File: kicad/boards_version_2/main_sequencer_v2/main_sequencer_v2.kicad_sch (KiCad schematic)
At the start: 33 parts

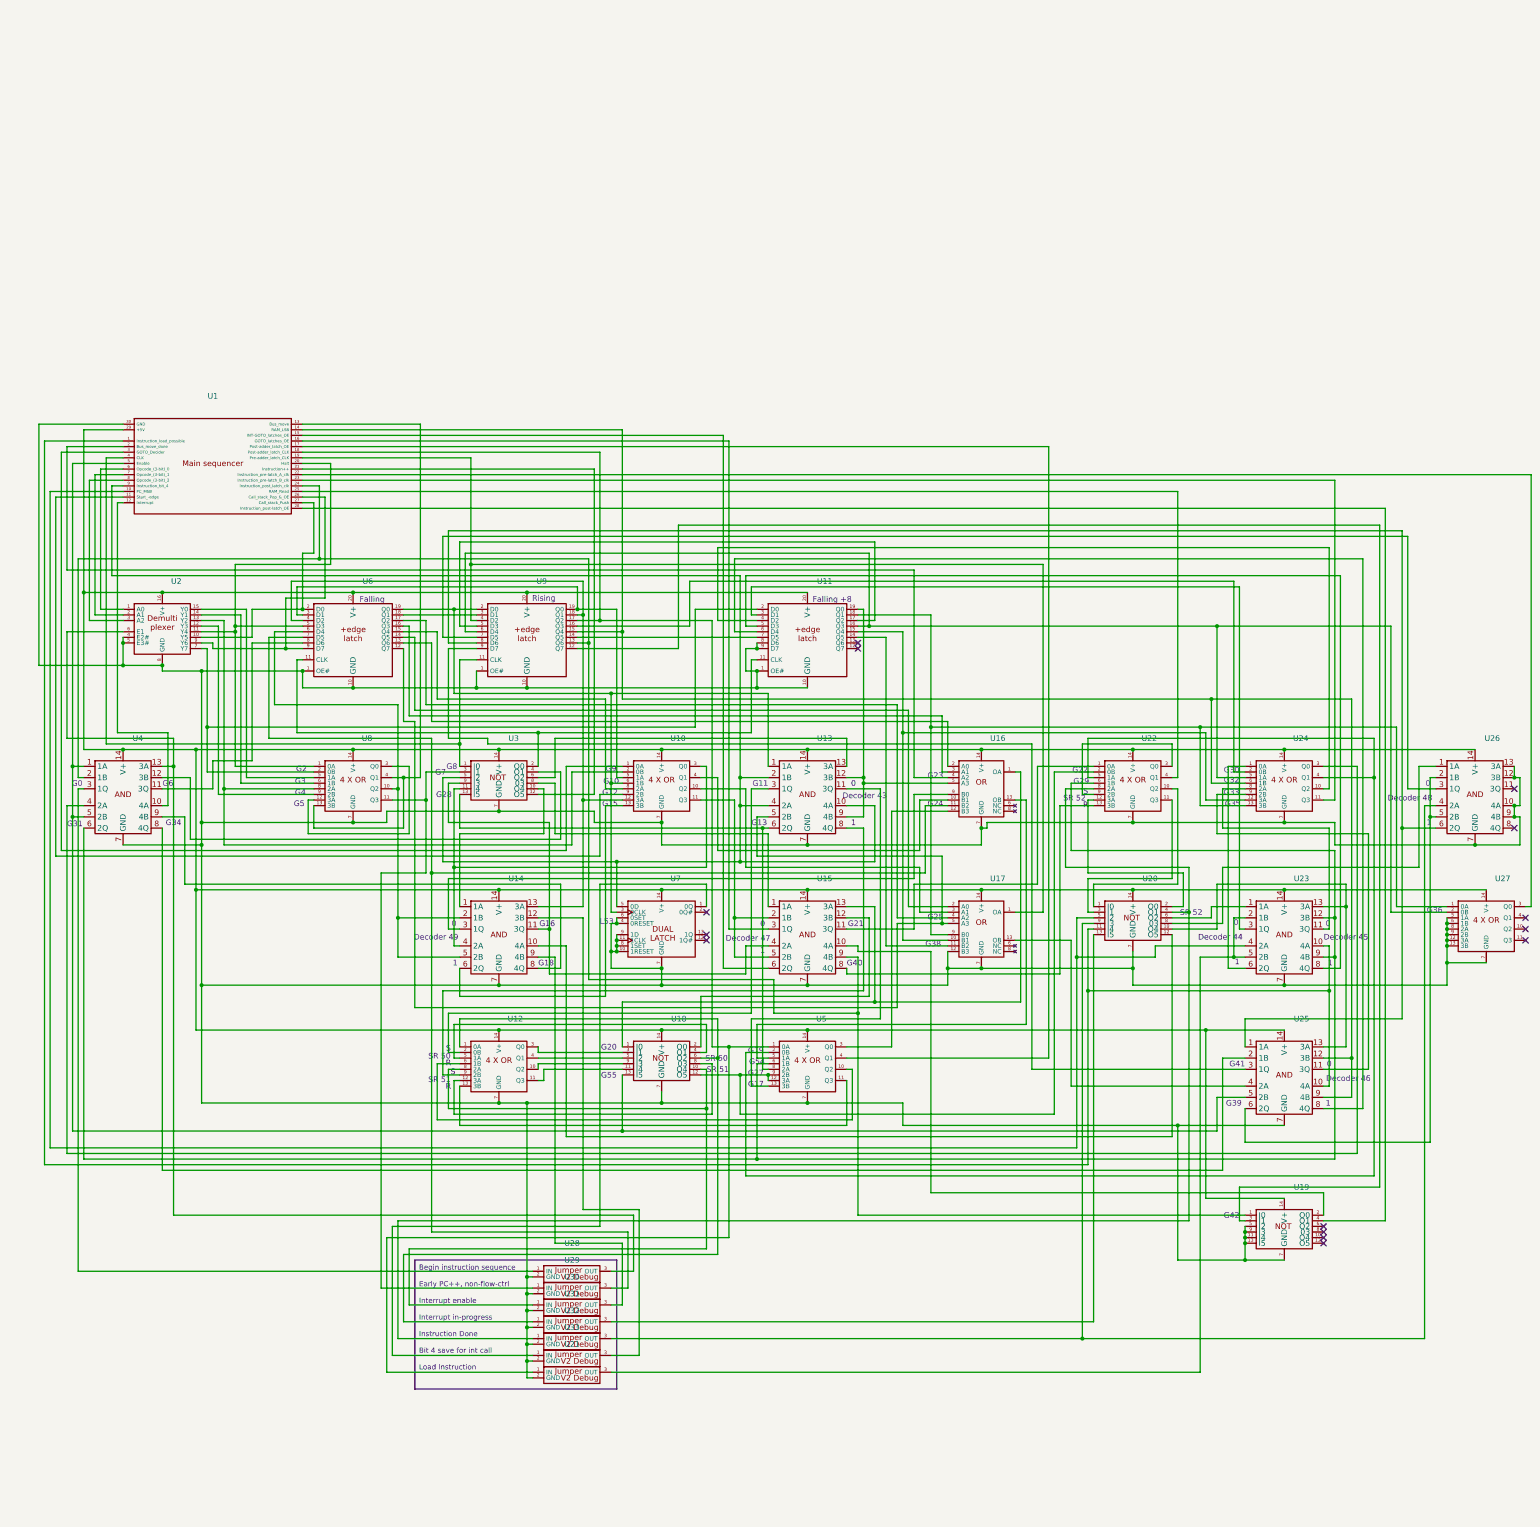
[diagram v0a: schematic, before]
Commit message: Debug figured out and work on ctrl unit main
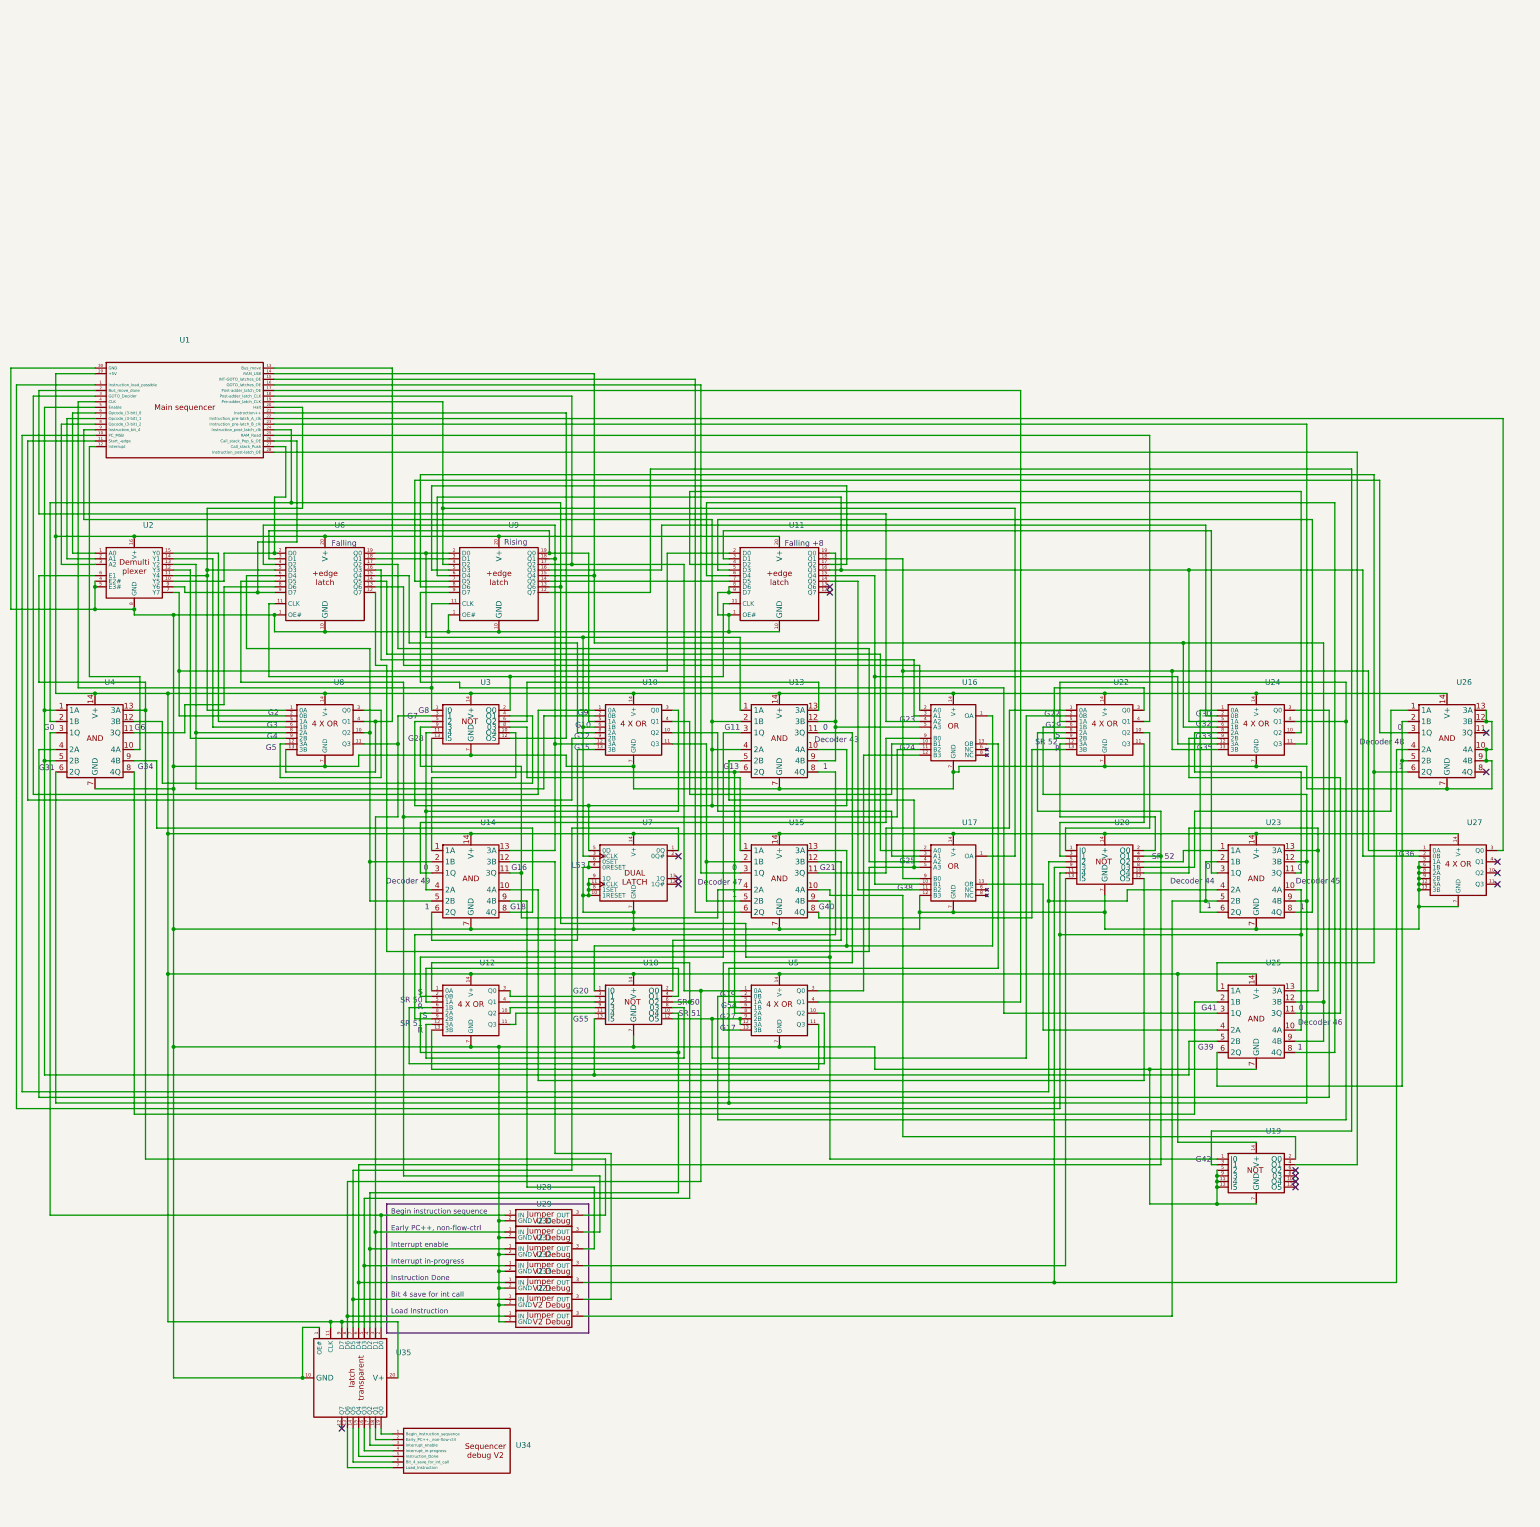
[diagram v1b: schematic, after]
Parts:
- added U34: ~, Connector_PinHeader_2.54mm:PinHeader_2x04_P2.54mm_Vertical, symbol custom_symbol_lib:debug_v2_sequencer
- added U35: ~, Package_DIP:DIP-20_W7.62mm, symbol custom_symbol_lib:8_bit_transparent_latch
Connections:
- net at U12.8 (2A), U18.10 (O4), U30.1 (IN): now also U35.4 (D2)
- net at U1.30 (GND), U10.7 (GND), U11.1 (OE#)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: now also U35.1 (OE#), U35.10 (GND)
- net at U33.1 (IN), U7.1 (0Q): now also U35.7 (D5)
- net at U1.29 (+5V), U10.14 (V+), U11.20 (V+)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: now also U35.11 (CLK), U35.20 (V+), U35.9 (D7)
- net at U28.1 (IN), U4.3 (1Q): now also U35.2 (D0)
- net at U12.1 (0A), U18.6 (O2), U31.1 (IN): now also U35.5 (D3)
- net at U29.1 (IN), U3.3 (I1), U8.11 (Q3): now also U35.3 (D1)
- net at U20.4 (O1), U22.8 (2A), U32.1 (IN): now also U35.6 (D4)
- net at U1.18 (Post-adder_latch_CLK), U21.1 (IN), U5.1 (0A)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: now also U35.8 (D6)
- new net: U34.1 (Begin_instruction_sequence), U35.19 (Q0)
- new net: U34.2 (Early_PC++,_non-flow-ctrl), U35.18 (Q1)
- new net: U34.3 (Interrupt_enable), U35.17 (Q2)
- new net: U34.4 (Interrupt_in-progress), U35.16 (Q3)
- new net: U34.5 (Instruction_Done), U35.15 (Q4)
- new net: U34.6 (Bit_4_save_for_int_call), U35.14 (Q5)
- new net: U34.7 (Load_Instruction), U35.13 (Q6)
- no-connect marks 14 -> 15
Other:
- moved on the sheet: U1, U10, U11, U12, U13, U14, U15, U16, U17, U18, U19, U2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

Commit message: Work mostly on bus
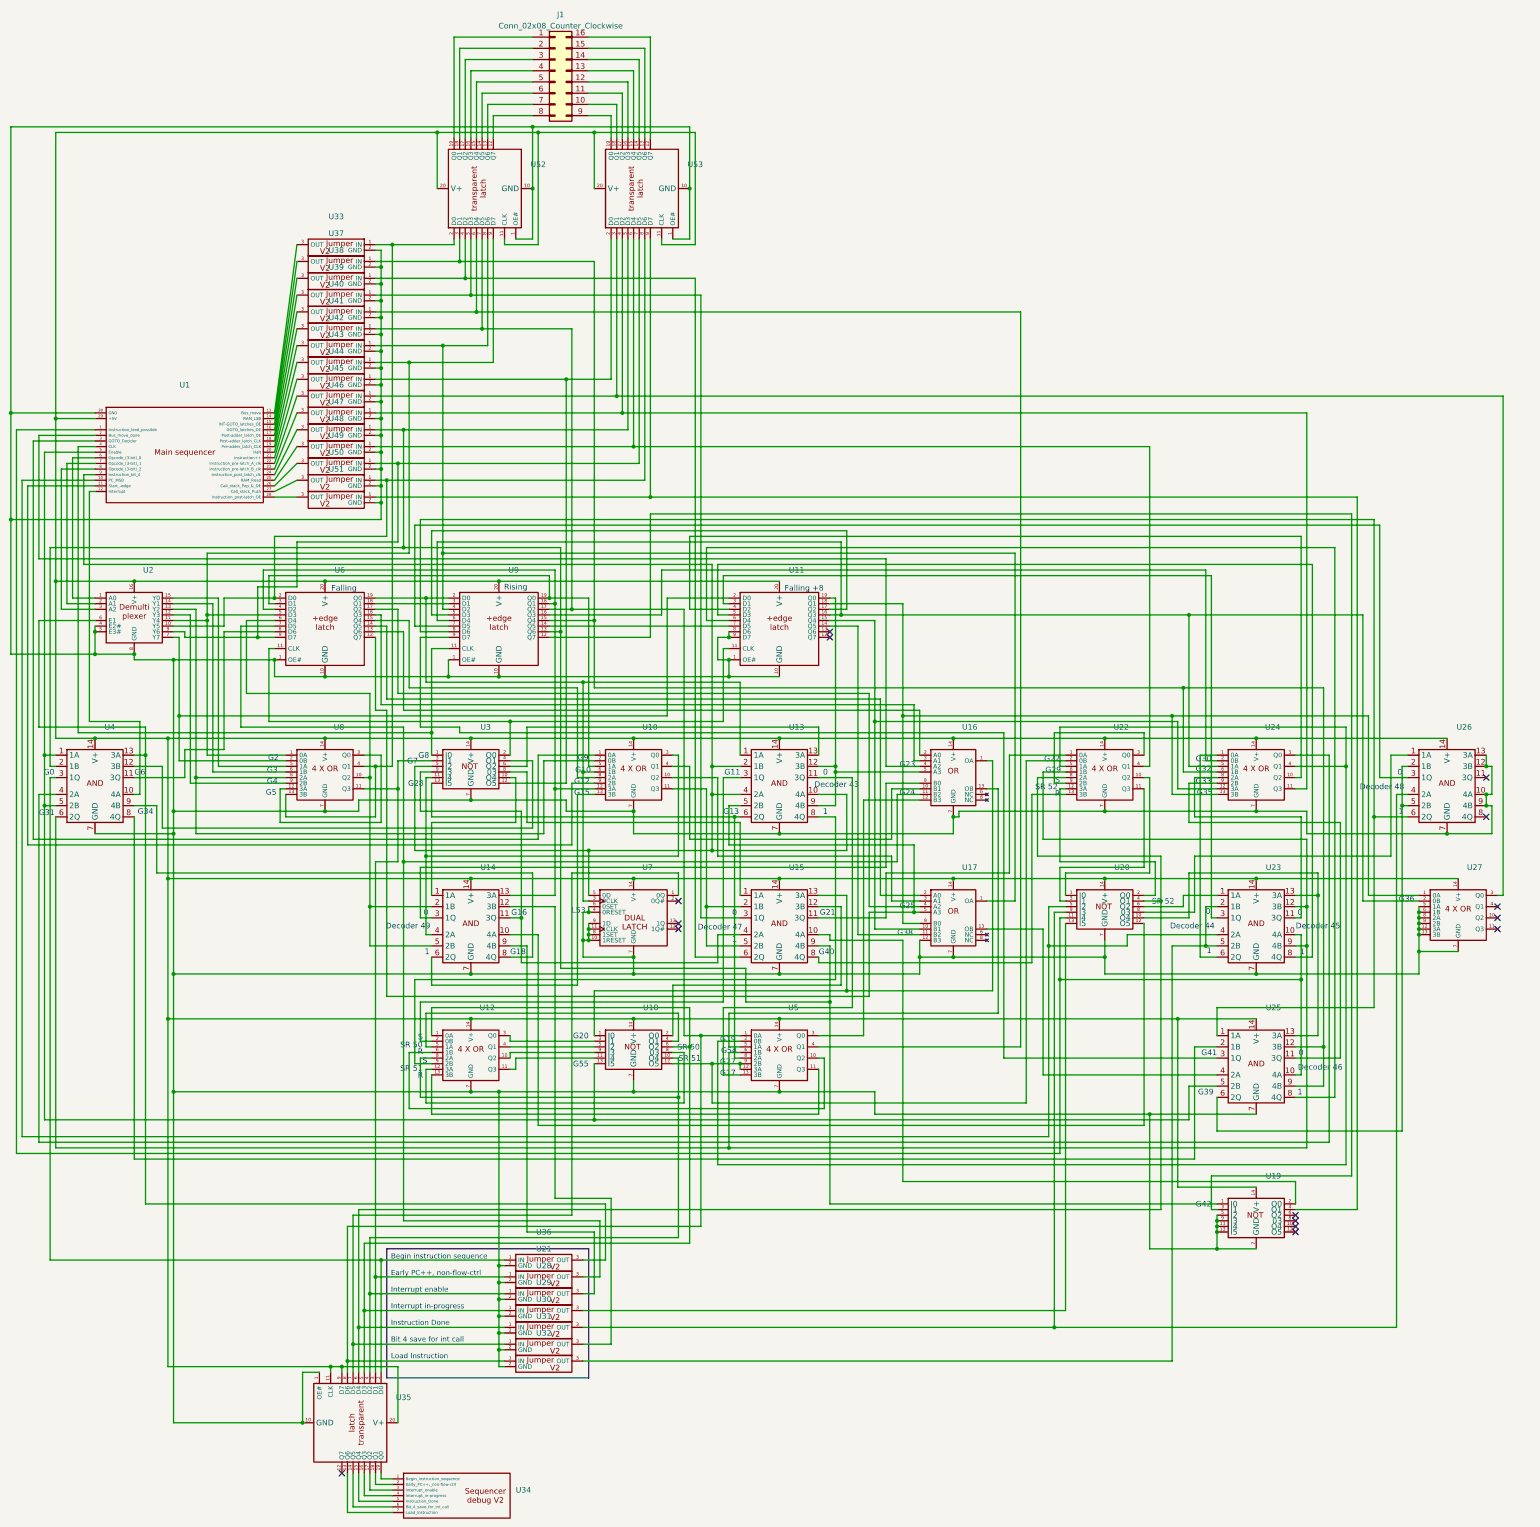
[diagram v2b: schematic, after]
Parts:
- removed U21, U28, U29, U30, U31, U32, U33: ~, custom_footprint_library:jumper_v2_gnd_debug_footprint, symbol custom_symbol_lib:jumper_v2_gnd_debug
- added J1: Conn_02x08_Counter_Clockwise, Connector_PinHeader_2.54mm:PinHeader_2x08_P2.54mm_Vertical, symbol Connector_Generic:Conn_02x08_Counter_Clockwise
- added U21, U28, U29, U30, U31, U32, U33, U36, U37, U38, U39, U40, U41, U42, U43, U44, U45, U46, U47, U48, U49, U50, U51: ~, custom_footprint_library:jumper_v2_gnd_footprint, symbol custom_symbol_lib:jumer_v2_gnd
- added U52, U53: ~, Package_DIP:DIP-20_W7.62mm, symbol custom_symbol_lib:8_bit_transparent_latch
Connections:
- net at U12.8 (2A), U18.10 (O4), U35.4 (D2): now also U28.1 (IN)
- net at U1.30 (GND), U10.7 (GND), U11.1 (OE#)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: now also U21.2 (GND), U28.2 (GND), U29.2 (GND), U30.2 (GND), U31.2 (GND), U32.2 (GND), U33.2 (GND), U36.2 (GND), U37.2 (GND), U38.2 (GND), U39.2 (GND), U40.2 (GND), U41.2 (GND), U42.2 (GND), U43.2 (GND), U44.2 (GND), U45.2 (GND), U46.2 (GND), U47.2 (GND), U48.2 (GND), U49.2 (GND), U50.2 (GND), U51.2 (GND), U52.1 (OE#), U52.10 (GND), U53.1 (OE#), U53.10 (GND)
- net at U14.9 (4B): now also U28.3 (OUT)
- net at U35.7 (D5), U7.1 (0Q): now also U31.1 (IN)
- net at U1.29 (+5V), U10.14 (V+), U11.20 (V+)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: now also U52.11 (CLK), U52.20 (V+), U53.11 (CLK), U53.20 (V+)
- net at U2.10 (Y5), U6.2 (D0): now also U50.1 (IN), U53.8 (D6); no longer U1.27 (Call_stack_Push)
- net at U2.11 (Y4), U6.5 (D3), U8.1 (0A): now also U43.1 (IN), U52.9 (D7); no longer U1.20 (Halt)
- net at U16.11 (B2), U6.7 (D5): now also U21.3 (OUT)
- net at U2.9 (Y6), U6.9 (D7): now also U49.1 (IN), U53.7 (D5); no longer U1.26 (Call_stack_Pop_&_OE)
- net at U2.6 (E1), U4.13 (3A): now also U36.3 (OUT)
- net at U15.9 (4B), U19.1 (I0), U4.2 (1B)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: now also U47.1 (IN), U53.5 (D3); no longer U1.24 (Instruction_post_latch_clk)
- net at U35.2 (D0), U4.3 (1Q): now also U36.1 (IN)
- net at U12.1 (0A), U18.6 (O2), U35.5 (D3): now also U29.1 (IN)
- net at U15.3 (1Q): now also U39.1 (IN), U52.5 (D3); no longer U1.16 (GOTO_latches_OE)
- net at U15.6 (2Q): now also U38.1 (IN), U52.4 (D2); no longer U1.15 (INT-GOTO_latches_OE)
- net at U24.6 (1B), U25.12 (3B), U25.9 (4B)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: now also U37.1 (IN), U52.3 (D1); no longer U1.14 (RAM_LSB)
- net at U3.3 (I1), U35.3 (D1), U8.11 (Q3): now also U21.1 (IN)
- net at U8.13 (3B), U8.4 (Q1): now also U33.1 (IN), U52.2 (D0); no longer U1.13 (Bus_move)
- net at U20.4 (O1), U22.8 (2A), U35.6 (D4): now also U30.1 (IN)
- net at U20.9 (I3), U26.4 (2A): now also U30.3 (OUT)
- net at U23.2 (1B), U23.5 (2B): now also U32.3 (OUT)
- net at U3.12 (O5): now also U44.1 (IN), U53.2 (D0); no longer U1.21 (Instruction++)
- net at U5.4 (Q1): now also U40.1 (IN), U52.6 (D4); no longer U1.17 (Post-adder_latch_OE)
- net at U35.8 (D6), U5.1 (0A), U9.17 (Q2): now also U32.1 (IN), U41.1 (IN), U52.7 (D5); no longer U1.18 (Post-adder_latch_CLK)
- net at U17.1 (OA), U9.4 (D2): now also U42.1 (IN), U52.8 (D6); no longer U1.19 (Pre-adder_latch_CLK)
- net at U27.3 (Q0): now also U45.1 (IN), U53.3 (D1); no longer U1.22 (Instruction_pre-latch_A_clk)
- net at U24.11 (Q3): now also U46.1 (IN), U53.4 (D2); no longer U1.23 (Instruction_pre-latch_B_clk)
- net at U22.4 (Q1): now also U48.1 (IN), U53.6 (D4); no longer U1.25 (RAM_Read)
- net at U19.4 (O1): now also U51.1 (IN), U53.9 (D7); no longer U1.28 (Instruction_post-latch_OE)
- net at U20.13 (I5): now also U29.3 (OUT)
- net at U14.12 (3B): now also U31.3 (OUT)
- new net: U1.24 (Instruction_post_latch_clk), U47.3 (OUT)
- new net: J1.1 (Pin_1), U52.19 (Q0)
- new net: J1.10 (Pin_10), U53.18 (Q1)
- new net: J1.11 (Pin_11), U53.17 (Q2)
- new net: J1.12 (Pin_12), U53.16 (Q3)
- new net: J1.13 (Pin_13), U53.15 (Q4)
- new net: J1.14 (Pin_14), U53.14 (Q5)
- new net: J1.15 (Pin_15), U53.13 (Q6)
- new net: J1.16 (Pin_16), U53.12 (Q7)
- new net: J1.2 (Pin_2), U52.18 (Q1)
- new net: J1.3 (Pin_3), U52.17 (Q2)
- new net: J1.4 (Pin_4), U52.16 (Q3)
- new net: J1.5 (Pin_5), U52.15 (Q4)
- new net: J1.6 (Pin_6), U52.14 (Q5)
- new net: J1.7 (Pin_7), U52.13 (Q6)
- new net: J1.8 (Pin_8), U52.12 (Q7)
- new net: J1.9 (Pin_9), U53.19 (Q0)
- new net: U1.23 (Instruction_pre-latch_B_clk), U46.3 (OUT)
- new net: U1.19 (Pre-adder_latch_CLK), U42.3 (OUT)
- new net: U1.14 (RAM_LSB), U37.3 (OUT)
- new net: U1.13 (Bus_move), U33.3 (OUT)
- new net: U1.22 (Instruction_pre-latch_A_clk), U45.3 (OUT)
- new net: U1.15 (INT-GOTO_latches_OE), U38.3 (OUT)
- new net: U1.16 (GOTO_latches_OE), U39.3 (OUT)
- new net: U1.17 (Post-adder_latch_OE), U40.3 (OUT)
- new net: U1.18 (Post-adder_latch_CLK), U41.3 (OUT)
- new net: U1.20 (Halt), U43.3 (OUT)
- new net: U1.21 (Instruction++), U44.3 (OUT)
- new net: U1.25 (RAM_Read), U48.3 (OUT)
- new net: U1.26 (Call_stack_Pop_&_OE), U49.3 (OUT)
- new net: U1.27 (Call_stack_Push), U50.3 (OUT)
- new net: U1.28 (Instruction_post-latch_OE), U51.3 (OUT)
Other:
- moved on the sheet: U1, U10, U11, U12, U13, U14, U15, U16, U17, U18, U19, U2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
